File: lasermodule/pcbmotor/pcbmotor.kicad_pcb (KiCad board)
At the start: 4 copper layers, 48.1 x 43.4 mm, 1 part, among them J1 Conn_01x03

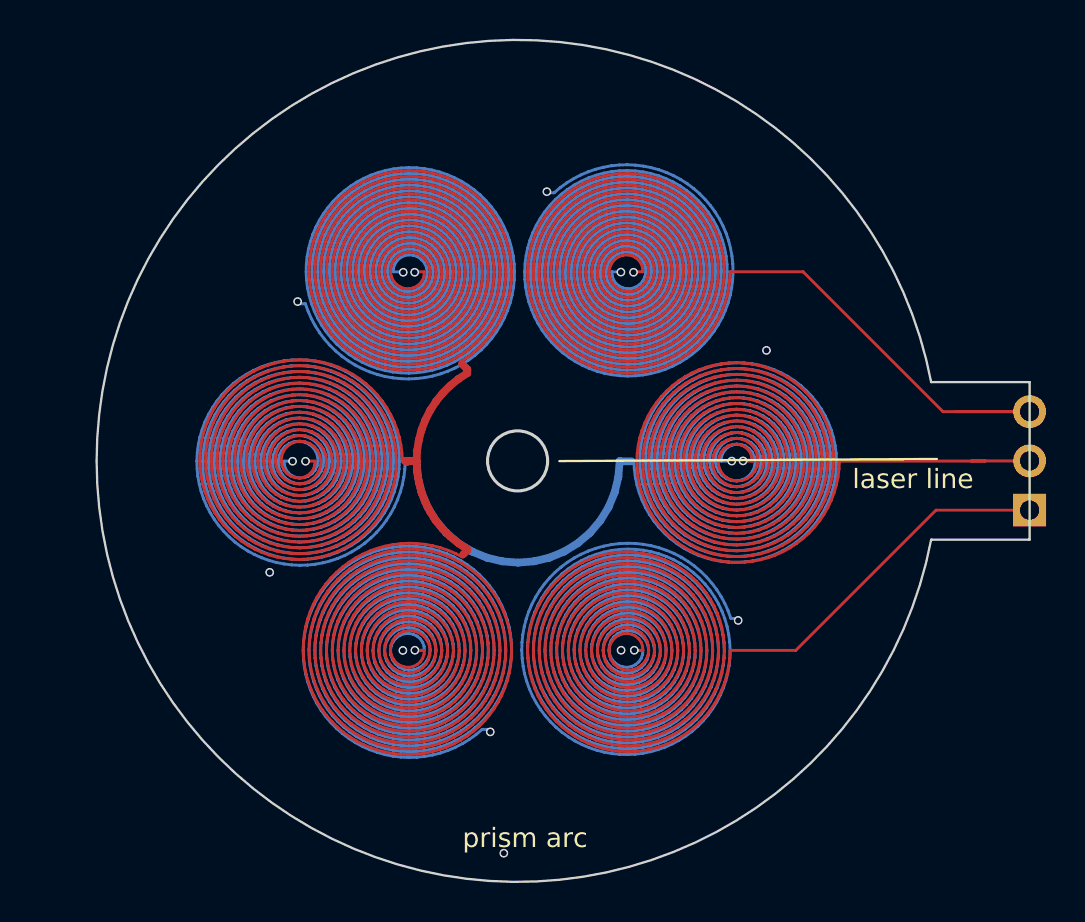
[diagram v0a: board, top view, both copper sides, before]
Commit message: further cleaned up and tested renders in blender
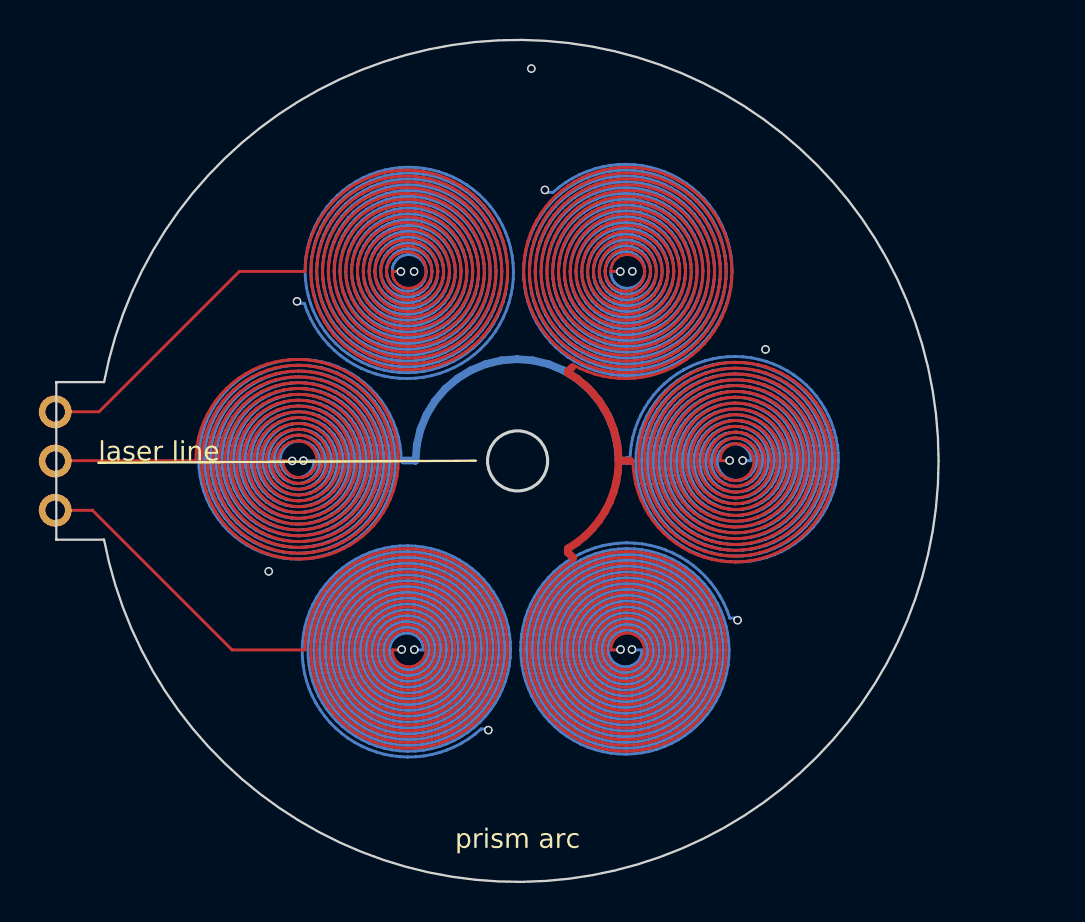
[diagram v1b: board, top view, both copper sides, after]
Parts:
- J1: footprint Connector_PinHeader_2.54mm:PinHeader_1x03_P2.54mm_Vertical -> pcbmotor:PinHeader_1x03_P2.54mm_Vertical
- moved J1 50.4 mm to (80.9, 114.1), turned to 180 degrees
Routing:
- net PH1: track 7450.6 -> 7439.4 mm
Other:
- board size 48.1 x 43.4 mm -> 45.5 x 43.4 mm
- board text added: "PCB3D_BR_motor"
- board text added: "PCB3D_TL_motor"
